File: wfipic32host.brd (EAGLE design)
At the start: 95.2 x 42.9 mm, 67 parts, among them IC1 BMA490L, IC2 TCAN330GD, IC3 WFI32E01PE-I, J1 MLE-105-01-G-DV, J2 MLE-105-01-G-DV, J3 MLE-105-01-G-DV, J4 MLE-105-01-G-DV, U1 PIC32MK0512MCJ048T-I/Y8XTQFP4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, U2 MAX6126B30

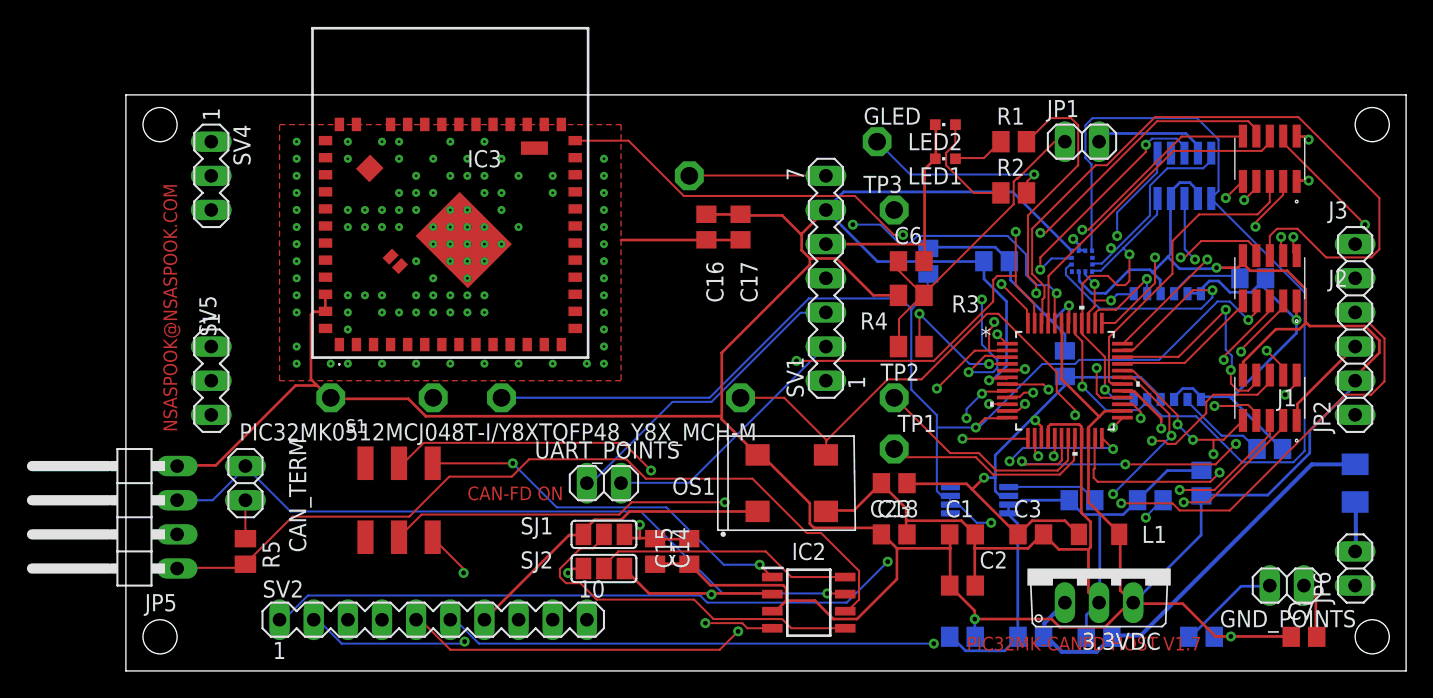
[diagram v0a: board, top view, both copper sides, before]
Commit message: up
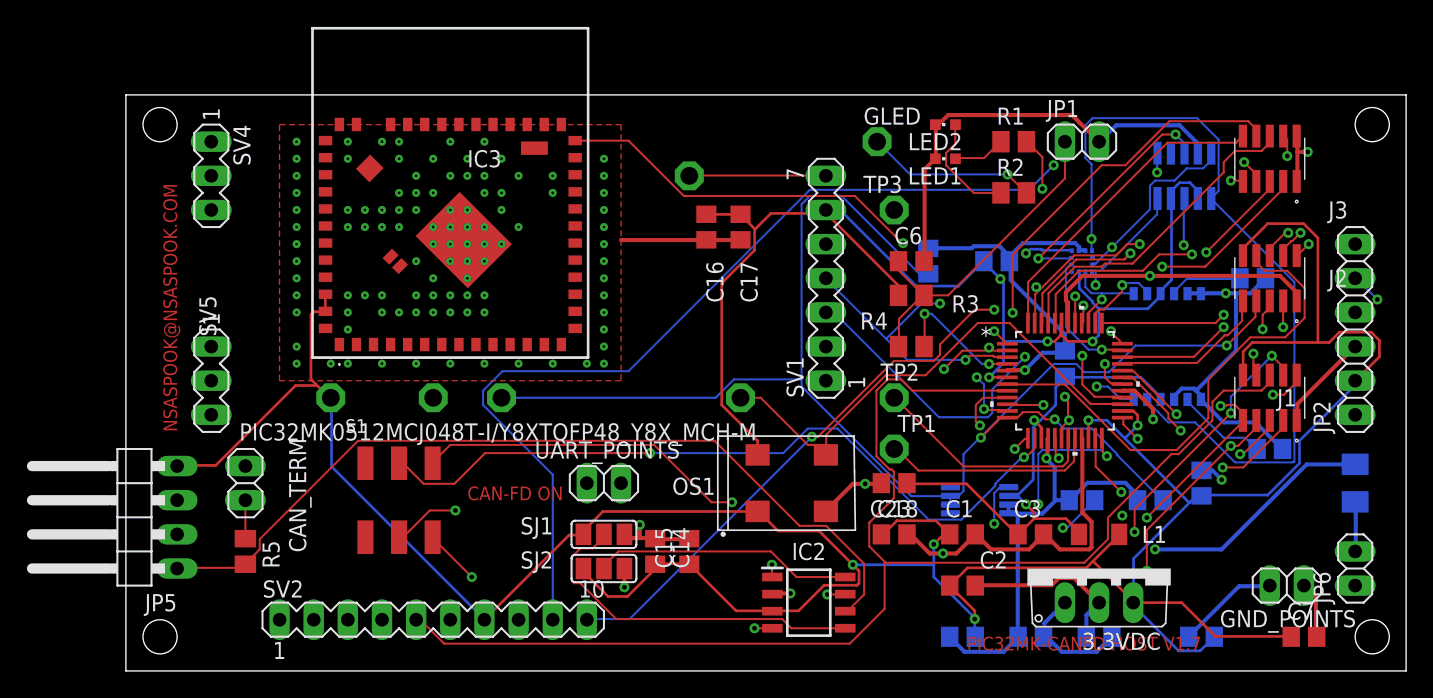
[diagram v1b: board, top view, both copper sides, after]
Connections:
- net VSS: now also IC3.55, IC3.56, IC3.57
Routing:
- net QEA2: track 84.0 -> 115.8 mm
- net PGC_C1RX: track 122.0 -> 90.7 mm, vias 2 -> 3
- net INDX2: track 54.1 -> 24.8 mm, vias 0 -> 2
- net VDD: track 369.8 -> 349.3 mm, vias 5 -> 10
- net DIS_CS: track 82.9 -> 101.7 mm, vias 4 -> 0
- net AN0: track 23.9 -> 40.2 mm
- net PGD_C1TX: track 103.4 -> 89.0 mm, vias 3 -> 2
- net EXT_SW2: track 24.0 -> 37.0 mm, vias 2 -> 0
- net VREF+: track 102.2 -> 112.3 mm, vias 4 -> 3
- net VSS: track 218.9 -> 228.6 mm, vias 111 -> 114
- net QEB2: track 79.8 -> 71.0 mm, vias 3 -> 5
- net MCLR_SIG: track 92.4 -> 100.4 mm
- net N$4: track 6.82 -> 14.2 mm, vias 0 -> 2
- net RED_LED: track 30.5 -> 23.2 mm
- net SCK1: track 99.4 -> 92.6 mm, vias 2 -> 3
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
